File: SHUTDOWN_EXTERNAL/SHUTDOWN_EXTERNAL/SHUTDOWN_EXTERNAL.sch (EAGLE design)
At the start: 15 parts

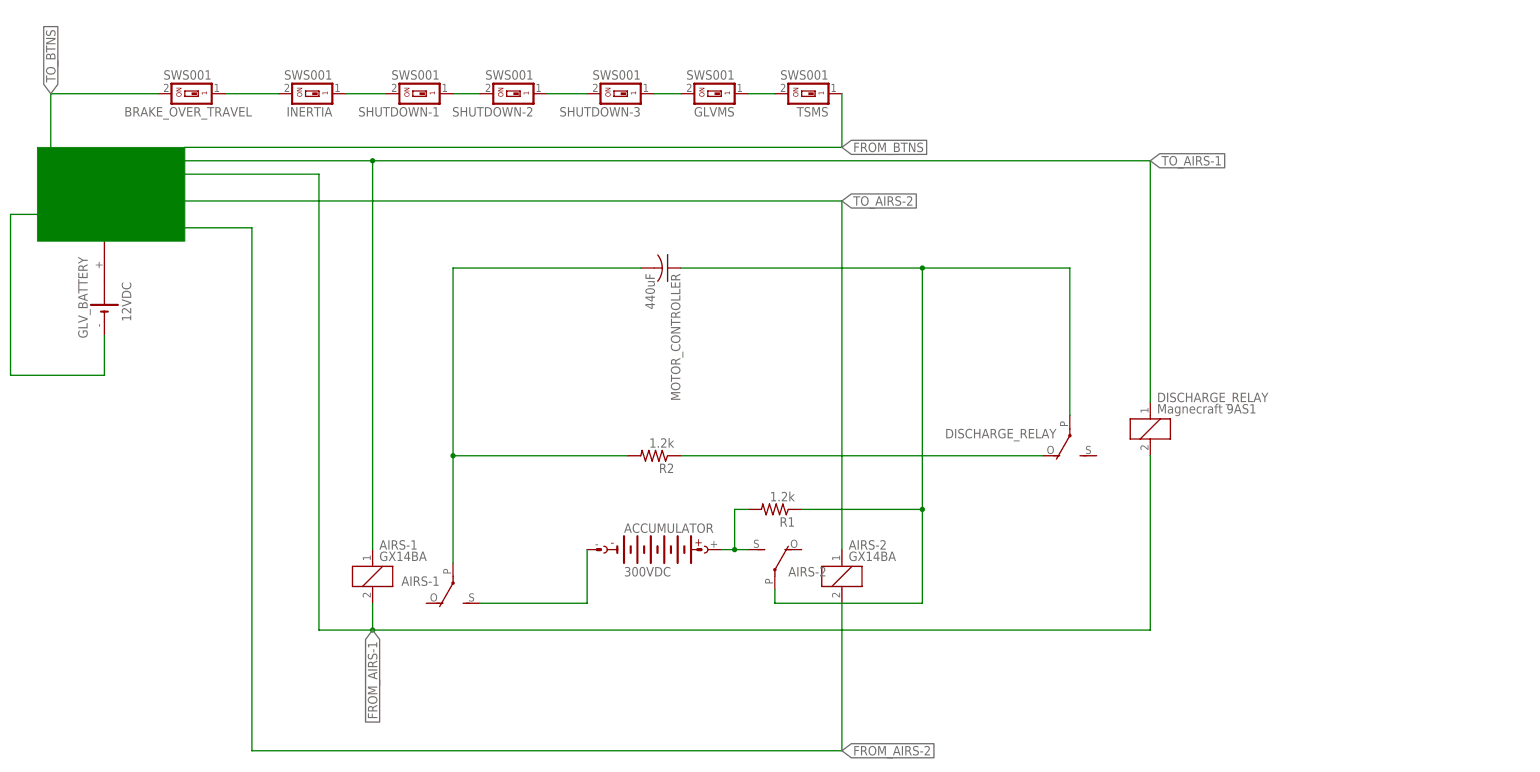
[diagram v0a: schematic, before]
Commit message: PCB Designs
Rev C
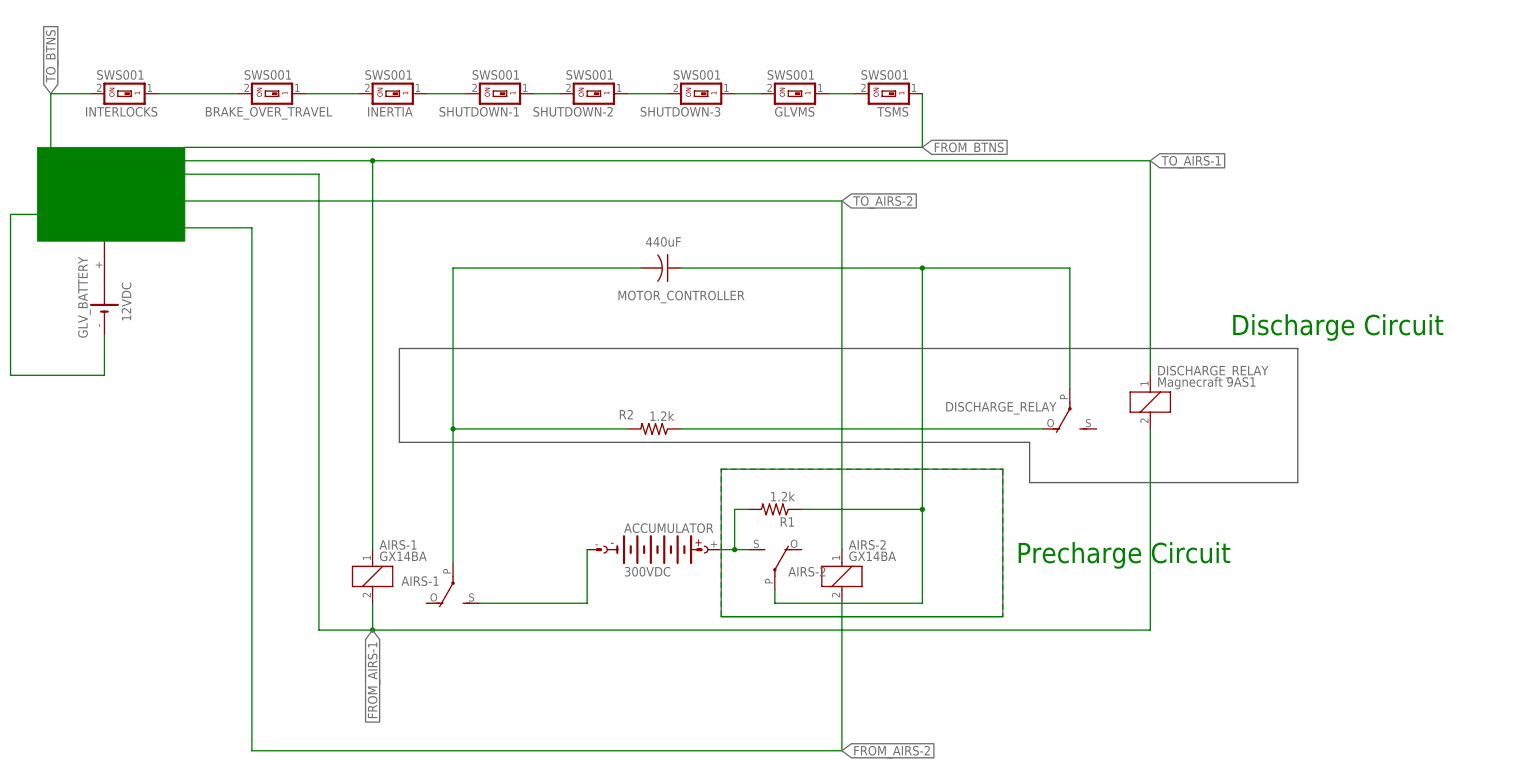
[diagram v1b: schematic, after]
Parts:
- added INTERLOCKS: SWS001, smd-special:SWS001
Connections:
- new net N$8: BRAKE_OVER_TRAVEL.2, INTERLOCKS.1
- net TO_BTNS: now also INTERLOCKS.2; no longer BRAKE_OVER_TRAVEL.2
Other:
- note added: "Discharge Circuit"
- note added: "Precharge Circuit"
- moved on the sheet: BRAKE_OVER_TRAVEL, DISCHARGE_RELAY, GLVMS, INERTIA, R2, SHUTDOWN-1, SHUTDOWN-2, SHUTDOWN-3, TSMS
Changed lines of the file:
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@@
 <part name="R1" library="rcl" library_urn="urn:adsk.eagle:library:334" deviceset="R-US_" device="0411/15" package3d_urn="urn:adsk.eagle:package:23568/1" value="1.2k"/>
 <part name="R2" library="rcl" library_urn="urn:adsk.eagle:library:334" deviceset="R-US_" device="0411/15" package3d_urn="urn:adsk.eagle:package:23568/1" value="1.2k"/>
+<part name="INTERLOCKS" library="smd-special" library_urn="urn:adsk.eagle:library:362" deviceset="SWS001" device="" package3d_urn="urn:adsk.eagle:package:26467/1"/>
 </parts>
 <sheets>
@@
 </polygon>
 <text x="-27.94" y="73.66" size="1.778" layer="88">SHUTDOWN CIRCUIT</text>
+<text x="154.94" y="5.08" size="3.81" layer="91">Precharge Circuit</text>
+<text x="195.58" y="48.26" size="3.81" layer="91">Discharge Circuit</text>
 </plain>
 <instances>
@@
 <attribute name="VALUE" x="-12.7" y="50.8" size="1.778" layer="96" rot="R90"/>
 </instance>
-<instance part="MOTOR_CONTROLLER" gate="G$1" x="88.9" y="60.96" rot="R270"/>
-<instance part="DISCHARGE_RELAY" gate="1" x="180.34" y="30.48"/>
-<instance part="DISCHARGE_RELAY" gate="2" x="165.1" y="30.48" rot="R180"/>
-<instance part="BRAKE_OVER_TRAVEL" gate="G$1" x="0" y="93.98" smashed="yes" rot="R90">
-<attribute name="NAME" x="10.16" y="91.44" size="1.778" layer="95" rot="R180"/>
-<attribute name="VALUE" x="2.54" y="98.425" size="1.778" layer="96" rot="R180"/>
-</instance>
-<instance part="INERTIA" gate="G$1" x="22.86" y="93.98" rot="R90"/>
-<instance part="SHUTDOWN-1" gate="G$1" x="43.18" y="93.98" rot="R90"/>
-<instance part="SHUTDOWN-2" gate="G$1" x="60.96" y="93.98" rot="R90"/>
-<instance part="SHUTDOWN-3" gate="G$1" x="81.28" y="93.98" rot="R90"/>
-<instance part="GLVMS" gate="G$1" x="99.06" y="93.98" rot="R90"/>
-<instance part="TSMS" gate="G$1" x="116.84" y="93.98" rot="R90"/>
+<instance part="MOTOR_CONTROLLER" gate="G$1" x="88.9" y="60.96" smashed="yes" rot="R270">
+<attribute name="NAME" x="79.375" y="54.864" size="1.778" layer="95"/>
+<attribute name="VALUE" x="84.709" y="65.024" size="1.778" layer="96"/>
+</instance>
+<instance part="DISCHARGE_RELAY" gate="1" x="180.34" y="35.56"/>
+<instance part="DISCHARGE_RELAY" gate="2" x="165.1" y="35.56" rot="R180"/>
+<instance part="BRAKE_OVER_TRAVEL" gate="G$1" x="15.24" y="93.98" smashed="yes" rot="R90">
+<attribute name="NAME" x="25.4" y="91.44" size="1.778" layer="95" rot="R180"/>
+<attribute name="VALUE" x="17.78" y="98.425" size="1.778" layer="96" rot="R180"/>
+</instance>
+<instance part="INERTIA" gate="G$1" x="38.1" y="93.98" rot="R90"/>
+<instance part="SHUTDOWN-1" gate="G$1" x="58.42" y="93.98" rot="R90"/>
+<instance part="SHUTDOWN-2" gate="G$1" x="76.2" y="93.98" rot="R90"/>
+<instance part="SHUTDOWN-3" gate="G$1" x="96.52" y="93.98" rot="R90"/>
+<instance part="GLVMS" gate="G$1" x="114.3" y="93.98" rot="R90"/>
+<instance part="TSMS" gate="G$1" x="132.08" y="93.98" rot="R90"/>
 <instance part="R1" gate="G$1" x="109.22" y="15.24" rot="R180"/>
-<instance part="R2" gate="G$1" x="86.36" y="25.4" rot="R180"/>
+<instance part="R2" gate="G$1" x="86.36" y="30.48" smashed="yes" rot="R180">
+<attribute name="NAME" x="82.55" y="34.0614" size="1.778" layer="95" rot="R180"/>
+<attribute name="VALUE" x="90.17" y="33.782" size="1.778" layer="96" rot="R180"/>
+</instance>
+<instance part="INTERLOCKS" gate="G$1" x="-12.7" y="93.98" smashed="yes" rot="R90">
+<attribute name="NAME" x="-7.62" y="91.44" size="1.778" layer="95" rot="R180"/>
+<attribute name="VALUE" x="-10.16" y="98.425" size="1.778" layer="96" rot="R180"/>
+</instance>
 </instances>
 <busses>
+<bus name="B$1">
+<segment>
+<wire x1="38.1" y1="45.72" x2="208.28" y2="45.72" width="0.762" layer="92"/>
+<wire x1="208.28" y1="45.72" x2="208.28" y2="20.32" width="0.762" layer="92"/>
+<wire x1="208.28" y1="20.32" x2="157.48" y2="20.32" width="0.762" layer="92"/>
+<wire x1="157.48" y1="20.32" x2="157.48" y2="27.94" width="0.762" layer="92"/>
+<wire x1="157.48" y1="27.94" x2="38.1" y2="27.94" width="0.762" layer="92"/>
+<wire x1="38.1" y1="27.94" x2="38.1" y2="45.72" width="0.762" layer="92"/>
+</segment>
+</bus>
+<bus name="B$2">
+<segment>
+<wire x1="99.06" y1="-5.08" x2="99.06" y2="22.86" width="0.762" layer="92"/>
+<wire x1="99.06" y1="22.86" x2="152.4" y2="22.86" width="0.762" layer="92"/>
+<wire x1="152.4" y1="22.86" x2="152.4" y2="-5.08" width="0.762" layer="92"/>
+<wire x1="152.4" y1="-5.08" x2="99.06" y2="-5.08" width="0.762" layer="92"/>
+</segment>
+</bus>
 </busses>
 <nets>
 <net name="TO_BTNS" class="0">
 <segment>
-<pinref part="BRAKE_OVER_TRAVEL" gate="G$1" pin="2"/>
-<wire x1="-7.62" y1="93.98" x2="-27.94" y2="93.98" width="0.1524" layer="91"/>
 <wire x1="-27.94" y1="93.98" x2="-27.94" y2="83.82" width="0.1524" layer="91"/>
 <label x="-27.94" y="93.98" size="1.778" layer="95" rot="R90" xref="yes"/>
+<pinref part="INTERLOCKS" gate="G$1" pin="2"/>
+<wire x1="-20.32" y1="93.98" x2="-27.94" y2="93.98" width="0.1524" layer="91"/>
 </segment>
 </net>
@@
 <pinref part="BRAKE_OVER_TRAVEL" gate="G$1" pin="1"/>
 <pinref part="INERTIA" gate="G$1" pin="2"/>
-<wire x1="5.08" y1="93.98" x2="15.24" y2="93.98" width="0.1524" layer="91"/>
+<wire x1="20.32" y1="93.98" x2="30.48" y2="93.98" width="0.1524" layer="91"/>
 </segment>
 </net>
@@
 <pinref part="INERTIA" gate="G$1" pin="1"/>
 <pinref part="SHUTDOWN-1" gate="G$1" pin="2"/>
-<wire x1="27.94" y1="93.98" x2="35.56" y2="93.98" width="0.1524" layer="91"/>
+<wire x1="43.18" y1="93.98" x2="50.8" y2="93.98" width="0.1524" layer="91"/>
 </segment>
 </net>
@@
 <pinref part="SHUTDOWN-1" gate="G$1" pin="1"/>
 <pinref part="SHUTDOWN-2" gate="G$1" pin="2"/>
-<wire x1="48.26" y1="93.98" x2="53.34" y2="93.98" width="0.1524" layer="91"/>
+<wire x1="63.5" y1="93.98" x2="68.58" y2="93.98" width="0.1524" layer="91"/>
 </segment>
 </net>
@@
 <pinref part="SHUTDOWN-2" gate="G$1" pin="1"/>
 <pinref part="SHUTDOWN-3" gate="G$1" pin="2"/>
-<wire x1="66.04" y1="93.98" x2="73.66" y2="93.98" width="0.1524" layer="91"/>
+<wire x1="81.28" y1="93.98" x2="88.9" y2="93.98" width="0.1524" layer="91"/>
 </segment>
 </net>
@@
 <pinref part="SHUTDOWN-3" gate="G$1" pin="1"/>
 <pinref part="GLVMS" gate="G$1" pin="2"/>
-<wire x1="86.36" y1="93.98" x2="91.44" y2="93.98" width="0.1524" layer="91"/>
+<wire x1="101.6" y1="93.98" x2="106.68" y2="93.98" width="0.1524" layer="91"/>
 </segment>
 </net>
@@
 <pinref part="GLVMS" gate="G$1" pin="1"/>
 <pinref part="TSMS" gate="G$1" pin="2"/>
-<wire x1="104.14" y1="93.98" x2="109.22" y2="93.98" width="0.1524" layer="91"/>
+<wire x1="119.38" y1="93.98" x2="124.46" y2="93.98" width="0.1524" layer="91"/>
 </segment>
 </net>
@@
 <segment>
 <pinref part="TSMS" gate="G$1" pin="1"/>
-<wire x1="121.92" y1="93.98" x2="121.92" y2="83.82" width="0.1524" layer="91"/>
-<wire x1="121.92" y1="83.82" x2="-2.54" y2="83.82" width="0.1524" layer="91"/>
-<label x="121.92" y="83.82" size="1.778" layer="95" xref="yes"/>
+<wire x1="137.16" y1="93.98" x2="137.16" y2="83.82" width="0.1524" layer="91"/>
+<wire x1="137.16" y1="83.82" x2="-2.54" y2="83.82" width="0.1524" layer="91"/>
+<label x="137.16" y="83.82" size="1.778" layer="95" xref="yes"/>
 </segment>
 </net>
@@
 <pinref part="DISCHARGE_RELAY" gate="1" pin="2"/>
 <wire x1="33.02" y1="-7.62" x2="180.34" y2="-7.62" width="0.1524" layer="91"/>
-<wire x1="180.34" y1="-7.62" x2="180.34" y2="25.4" width="0.1524" layer="91"/>
+<wire x1="180.34" y1="-7.62" x2="180.34" y2="30.48" width="0.1524" layer="91"/>
 </segment>
 </net>
@@
 <junction x="33.02" y="81.28"/>
 <pinref part="DISCHARGE_RELAY" gate="1" pin="1"/>
-<wire x1="180.34" y1="35.56" x2="180.34" y2="81.28" width="0.1524" layer="91"/>
+<wire x1="180.34" y1="40.64" x2="180.34" y2="81.28" width="0.1524" layer="91"/>
 <wire x1="180.34" y1="81.28" x2="33.02" y2="81.28" width="0.1524" layer="91"/>
 <label x="180.34" y="81.28" size="1.778" layer="95" xref="yes"/>
@@
 <junction x="137.16" y="15.24"/>
 <pinref part="DISCHARGE_RELAY" gate="2" pin="P"/>
-<wire x1="165.1" y1="33.02" x2="165.1" y2="60.96" width="0.1524" layer="91"/>
+<wire x1="165.1" y1="38.1" x2="165.1" y2="60.96" width="0.1524" layer="91"/>
 <wire x1="165.1" y1="60.96" x2="137.16" y2="60.96" width="0.1524" layer="91"/>
 <junction x="137.16" y="60.96"/>
@@
 <wire x1="83.82" y1="60.96" x2="48.26" y2="60.96" width="0.1524" layer="91"/>
 <pinref part="AIRS-1" gate="2" pin="P"/>
-<wire x1="48.26" y1="60.96" x2="48.26" y2="25.4" width="0.1524" layer="91"/>
+<wire x1="48.26" y1="60.96" x2="48.26" y2="30.48" width="0.1524" layer="91"/>
 <pinref part="R2" gate="G$1" pin="2"/>
-<wire x1="48.26" y1="25.4" x2="48.26" y2="5.08" width="0.1524" layer="91"/>
-<wire x1="81.28" y1="25.4" x2="48.26" y2="25.4" width="0.1524" layer="91"/>
-<junction x="48.26" y="25.4"/>
+<wire x1="48.26" y1="30.48" x2="48.26" y2="5.08" width="0.1524" layer="91"/>
+<wire x1="81.28" y1="30.48" x2="48.26" y2="30.48" width="0.1524" layer="91"/>
+<junction x="48.26" y="30.48"/>
 </segment>
 </net>
@@
 <pinref part="R2" gate="G$1" pin="1"/>
 <pinref part="DISCHARGE_RELAY" gate="2" pin="O"/>
-<wire x1="91.44" y1="25.4" x2="160.02" y2="25.4" width="0.1524" layer="91"/>
+<wire x1="91.44" y1="30.48" x2="160.02" y2="30.48" width="0.1524" layer="91"/>
 </segment>
 </net>
@@
 </segment>
 </net>
+<net name="N$8" class="0">
+<segment>
+<pinref part="INTERLOCKS" gate="G$1" pin="1"/>
+<pinref part="BRAKE_OVER_TRAVEL" gate="G$1" pin="2"/>
+<wire x1="-7.62" y1="93.98" x2="7.62" y2="93.98" width="0.1524" layer="91"/>
+</segment>
+</net>
+<net name="N$9" class="0">
+<segment>
+<wire x1="99.06" y1="-5.08" x2="99.06" y2="22.86" width="0.508" layer="91" style="longdash"/>
+<wire x1="99.06" y1="22.86" x2="152.4" y2="22.86" width="0.508" layer="91" style="longdash"/>
+<wire x1="152.4" y1="22.86" x2="152.4" y2="-5.08" width="0.508" layer="91" style="longdash"/>
+<wire x1="152.4" y1="-5.08" x2="99.06" y2="-5.08" width="0.1524" layer="91"/>
+</segment>
+</net>
